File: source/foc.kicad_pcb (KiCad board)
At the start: 2 copper layers, 68.4 x 79 mm, 208 parts, among them J1 Conn_01x04_Male, J2 TYPE-C-31-M-12, P1 SWD, Q1 NCEP60T20, Q10 CSD19536KCS, Q11 CSD19536KCS, Q12 CSD19536KCS, Q2 CSD19536KCS, Q3 CSD19536KCS, Q4 CSD19536KCS, Q5 CSD19536KCS, Q6 CSD19536KCS, Q7 CSD19536KCS, Q8 CSD19536KCS, Q9 CSD19536KCS, U1 BMI160, U10 HT7550, U11 STM32F405RGT6, U12 AMS1117-3.3, U2 IRS21867S, U3 IRS21867S, U4 IRS21867S, U5 TX4130L/PW2902, U6 MS8311, U7 MS8311, U8 MS8311, U9 TJA1050T/CM,118, Y1 8MHz Crystal Resonator, X5032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

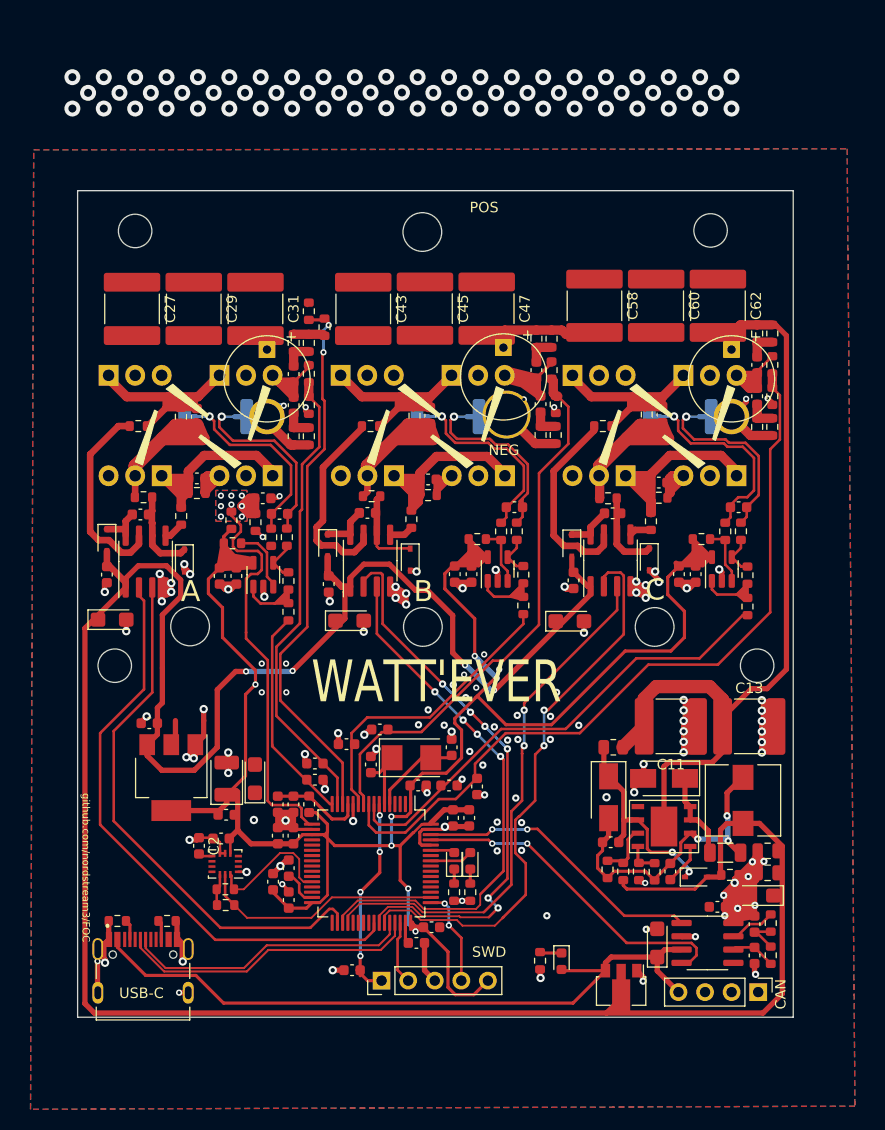
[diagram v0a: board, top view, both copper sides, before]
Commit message: Add files via upload
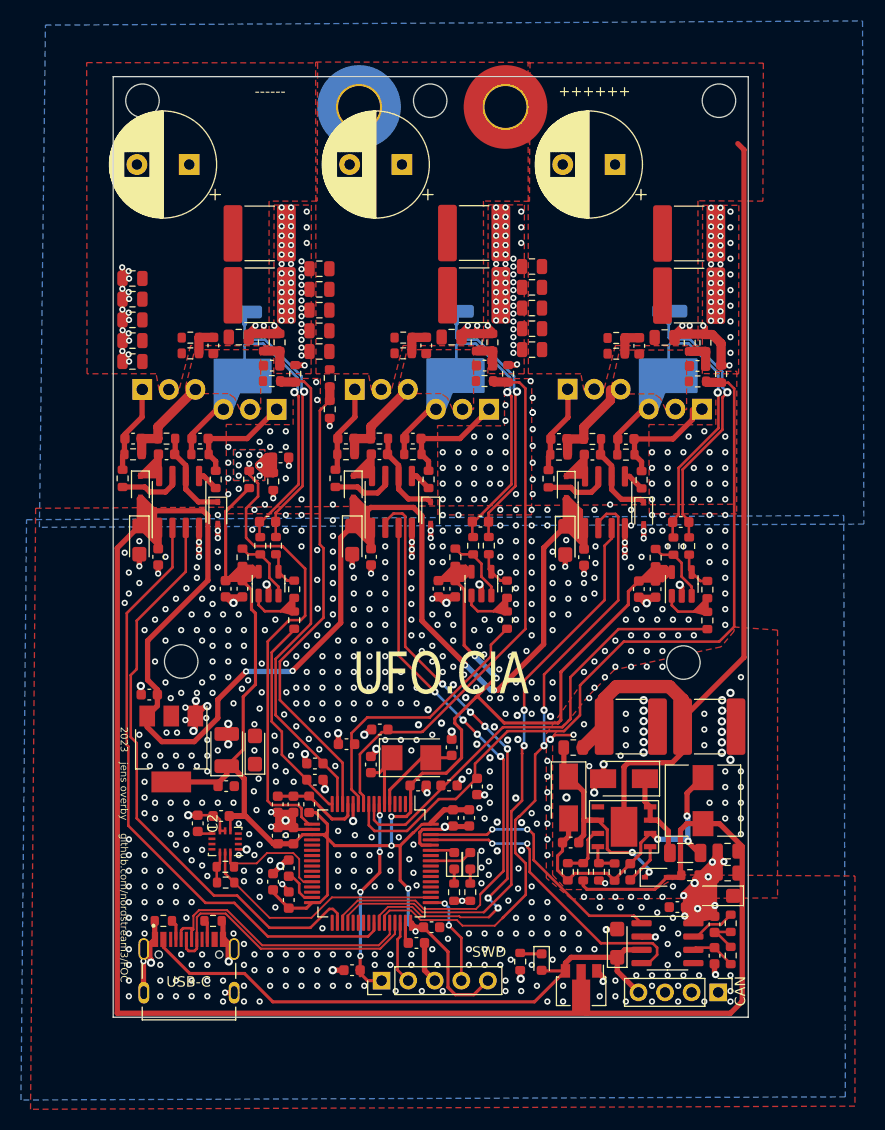
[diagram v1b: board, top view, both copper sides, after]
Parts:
- removed the C21 at (73.7, 108.8)
- removed the C22 at (75.3, 108.8)
- removed the C26 at (79.4, 102.9)
- removed the C31 at (77.1, 83.3)
- removed the C33 at (78.2, 87.5)
- removed the C40 at (93.8, 93.5)
- removed the C41 at (93.6, 99.6)
- removed the C58 at (109.5, 83.0)
- removed the H2 at (115.2, 113.7)
- removed the H4 at (70.8, 113.7)
- removed H8: MountingHole, MountingHole:MountingHole_3.7mm
- removed Q10, Q11, Q12, Q7, Q8, Q9: CSD19536KCS, Package_TO_SOT_THT:TO-220-3_Vertical
- removed the R21 at (80.2, 112.2)
- removed the R24 at (80.2, 109.3)
- removed the R25 at (74.9, 105.7)
- removed the R28 at (78.6, 105.1)
- removed the R29 at (80.1, 105.1)
- removed the U6 at (77.8, 108.7)
- added C27: 100n 100V, Capacitor_SMD:C_0805_2012Metric, F.Cu at (75.5, 86.0)
- added C28: 100n 100V, Capacitor_SMD:C_0805_2012Metric, F.Cu at (65.3, 88.3)
- added C29: 100n 100V, Capacitor_SMD:C_0805_2012Metric, F.Cu at (65.3, 86.3)
- added C30: 100n 100V, Capacitor_SMD:C_0805_2012Metric, F.Cu at (65.3, 80.4)
- added C32: 100n 100V, Capacitor_SMD:C_0805_2012Metric, F.Cu at (65.3, 82.4)
- added C34: 100n 100V, Capacitor_SMD:C_0805_2012Metric, F.Cu at (65.3, 84.3)
- added C35: 470u 80V, Capacitor_THT:CP_Radial_D10.0mm_P5.00mm, F.Cu at (70.8, 69.5)
- added C38: 2.2u, Capacitor_SMD:C_0603_1608Metric, F.Cu at (94.6, 110.0)
- added C39: 100n, Capacitor_SMD:C_0603_1608Metric, F.Cu at (96.2, 110.0)
- added C42: 2.2nF, Capacitor_SMD:C_0603_1608Metric, F.Cu at (85.7, 95.7)
- added C44: 100p, Capacitor_SMD:C_0603_1608Metric, F.Cu at (98.6, 103.6)
- added C46: 100n 100V, Capacitor_SMD:C_0805_2012Metric, F.Cu at (83.2, 87.4)
- added C48: 100n 100V, Capacitor_SMD:C_0805_2012Metric, F.Cu at (83.2, 79.5)
- added C54: 4.7n, Capacitor_SMD:C_0603_1608Metric, F.Cu at (93.4, 86.8)
- added C59: 2.2nF, Capacitor_SMD:C_0603_1608Metric, F.Cu at (106.1, 95.7)
- added C61: 100p, Capacitor_SMD:C_0603_1608Metric, F.Cu at (117.8, 103.7)
- added C63: 100n 100V, Capacitor_SMD:C_0805_2012Metric, F.Cu at (103.5, 85.2)
- added C67: 100n 100V, Capacitor_SMD:C_0805_2012Metric, F.Cu at (103.5, 81.2)
- added C68: 10u @ 100V, Capacitor_SMD:C_2220_5650Metric, F.Cu at (118.6, 76.1)
- added C69: 100n 100V, Capacitor_SMD:C_0805_2012Metric, F.Cu at (103.5, 83.2)
- added C70: 470u 80V, Capacitor_THT:CP_Radial_D10.0mm_P5.00mm, F.Cu at (111.5, 69.5)
- added C71: 4.7n, Capacitor_SMD:C_0603_1608Metric, F.Cu at (113.8, 86.8)
- added C72: 4.7n, Capacitor_SMD:C_0603_1608Metric, F.Cu at (119.4, 88.8)
- added H3: MountingHole, MountingHole:MountingHole_3.2mm_M3, F.Cu at (93.8, 63.4)
- added H7: MountingHole_Pad, MountingHole:MountingHole_4mm_Pad_TopOnly, F.Cu at (87.0, 64.0)
- added R35: 30k, Resistor_SMD:R_0603_1608Metric, F.Cu at (101.1, 113.0)
- added R39: 30k, Resistor_SMD:R_0603_1608Metric, F.Cu at (101.1, 110.1)
- added R41: 62k, Resistor_SMD:R_0603_1608Metric, F.Cu at (96.2, 107.0)
- added R44: 1k, Resistor_SMD:R_0603_1608Metric, F.Cu at (97.9, 105.9)
- added R45: 1k, Resistor_SMD:R_0603_1608Metric, F.Cu at (99.4, 105.9)
- added U7: MS8311, Package_TO_SOT_SMD:TSOT-23-5, F.Cu at (98.7, 109.6)
- C43, C60: value 10u @ 100V -> 2.2nF; footprint Capacitor_SMD:C_2220_5650Metric -> Capacitor_SMD:C_0603_1608Metric
- C45, C47, C62: value 10u @ 100V -> 100n 100V; footprint Capacitor_SMD:C_2220_5650Metric -> Capacitor_SMD:C_0805_2012Metric
- C49: value 470u 80V -> 10u @ 100V; footprint Custom:CP_Radial_D8.0mm_P5.00mm -> Capacitor_SMD:C_2220_5650Metric
- C50, C65: value 4.7n -> 100n 100V; footprint Capacitor_SMD:C_0603_1608Metric -> Capacitor_SMD:C_0805_2012Metric
- C51, C66: value 4.7n -> 10u @ 100V; footprint Capacitor_SMD:C_0603_1608Metric -> Capacitor_SMD:C_2220_5650Metric
- C52: value 2.2u -> 100n 100V; footprint Capacitor_SMD:C_0603_1608Metric -> Capacitor_SMD:C_0805_2012Metric
- C53: value 100n -> 470u 80V; footprint Capacitor_SMD:C_0603_1608Metric -> Capacitor_THT:CP_Radial_D10.0mm_P5.00mm
- C55: value 2.2nF -> 4.7n
- C56: value 2.2nF -> 2.2u
- C57: value 100p -> 100n
- C64: value 470u 80V -> 100n 100V; footprint Custom:CP_Radial_D8.0mm_P5.00mm -> Capacitor_SMD:C_0805_2012Metric
- H6: value MountingHole -> MountingHole_Pad; footprint MountingHole:MountingHole_3.7mm -> MountingHole:MountingHole_4mm_Pad_TopOnly
- moved H6 50.3 mm to (101.0, 64.0)
- moved C53 48.2 mm to (91.1, 69.5), turned to 180 degrees
- moved C52 42.6 mm to (83.2, 83.4), turned to 180 degrees
- moved Q4 31.9 mm to (99.4, 92.9)
- moved Q6 30.1 mm to (119.8, 92.9)
- moved C26 23.6 mm to (78.3, 103.6)
- moved Q3 23.6 mm to (86.6, 91.0)
- moved C65 23.5 mm to (103.5, 79.2), turned to 180 degrees
- moved R28 23.1 mm to (77.6, 105.9)
- moved R29 23.1 mm to (79.1, 105.9)
- moved R25 22.5 mm to (75.9, 107.0), turned to -90 degrees
- moved C50 22.1 mm to (83.2, 81.4), turned to 180 degrees
- moved C21 21.9 mm to (74.2, 110.1)
- moved C22 21.9 mm to (75.8, 110.1)
- moved R21 21.9 mm to (80.8, 113.0)
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- renumbered C36 to C21, C37 to C22, C42 to C26, C27 to C31, C29 to C33, C34 to C36, C35 to C37, C38 to C40, C39 to C41, C54 to C58, C67 to C73, C68 to C74, C69 to C75, C70 to C76, C71 to C77, C72 to C78, C73 to C79, C74 to C80, C75 to C81, C76 to C82, C77 to C83, C78 to C84, C79 to C85, C80 to C86, C81 to C87, C82 to C88, C83 to C89, C84 to C90, C85 to C91, C86 to C92, C87 to C93, C88 to C94, C89 to C95, C90 to C96, H3 to H2, H7 to H4, R35 to R21, R39 to R24, R41 to R25, R44 to R28, R45 to R29, U7 to U6
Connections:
- C26 pad 1: Net-(C42-Pad1) -> Net-(C26-Pad1)
- C26 pad 2: Net-(C42-Pad2) -> Net-(C26-Pad2)
- C43 pad 1: GND -> Net-(C43-Pad1)
- C43 pad 2: V_IN -> Net-(C43-Pad2)
- C45 pad 1: GND -> V_IN
- C45 pad 2: V_IN -> GND
- C47 pad 1: GND -> V_IN
- C47 pad 2: V_IN -> GND
- C49 pad 1: V_IN -> GND
- C49 pad 2: GND -> V_IN
- C50 pad 1: /driver/HS2 -> V_IN
- C50 pad 2: Net-(C50-Pad2) -> GND
- C51 pad 1: /driver/HS2 -> GND
- C51 pad 2: Net-(C51-Pad2) -> V_IN
- C52 pad 1: VCC -> V_IN
- C53 pad 1: VCC -> V_IN
- C55 pad 1: Net-(C55-Pad1) -> /driver/HS2
- C55 pad 2: /driver/HS3 -> Net-(C55-Pad2)
- C56 pad 1: Net-(C56-Pad1) -> VCC
- C56 pad 2: Net-(C56-Pad2) -> GND
- C57 pad 1: Net-(C57-Pad1) -> VCC
- C57 pad 2: Net-(C57-Pad2) -> GND
- C60 pad 1: GND -> Net-(C60-Pad1)
- C60 pad 2: V_IN -> Net-(C60-Pad2)
- C62 pad 1: GND -> V_IN
- C62 pad 2: V_IN -> GND
- C65 pad 1: /driver/HS3 -> V_IN
- C65 pad 2: Net-(C65-Pad2) -> GND
- C66 pad 1: /driver/HS3 -> GND
- C66 pad 2: Net-(C66-Pad2) -> V_IN
- NT3 pad 1: Net-(C42-Pad2) -> Net-(C44-Pad2)
- NT3 pad 2: Net-(C41-Pad2) -> Net-(C43-Pad2)
- NT4 pad 1: Net-(C42-Pad1) -> Net-(C44-Pad1)
- NT5 pad 1: Net-(C57-Pad2) -> Net-(C61-Pad2)
- NT5 pad 2: Net-(C56-Pad2) -> Net-(C60-Pad2)
- NT6 pad 1: Net-(C57-Pad1) -> Net-(C61-Pad1)
- Q3 pad 1: Net-(C24-Pad1) -> Net-(C42-Pad1)
- Q3 pad 3: /driver/HS1 -> /driver/HS2
- Q4 pad 1: Net-(C25-Pad1) -> Net-(C43-Pad1)
- Q4 pad 2: /driver/HS1 -> /driver/HS2
- Q4 pad 3: Net-(C25-Pad2) -> Net-(C43-Pad2)
- Q5 pad 1: Net-(C40-Pad1) -> Net-(C59-Pad1)
- Q5 pad 3: /driver/HS2 -> /driver/HS3
- Q6 pad 1: Net-(C41-Pad1) -> Net-(C60-Pad1)
- Q6 pad 2: /driver/HS2 -> /driver/HS3
- Q6 pad 3: Net-(C41-Pad2) -> Net-(C60-Pad2)
- R21 pad 2: /mcu/CURRENT_2 -> /mcu/CURRENT_1
- R28 pad 1: Net-(C42-Pad2) -> Net-(C26-Pad2)
- R29 pad 1: Net-(C42-Pad1) -> Net-(C26-Pad1)
- R37 pad 2: Net-(C40-Pad1) -> Net-(C42-Pad1)
- R38 pad 2: Net-(C41-Pad1) -> Net-(C43-Pad1)
- R42 pad 2: Net-(C40-Pad1) -> Net-(C42-Pad1)
- R43 pad 1: Net-(C41-Pad2) -> Net-(C43-Pad2)
- R43 pad 2: Net-(C41-Pad1) -> Net-(C43-Pad1)
- R46 pad 1: Net-(C41-Pad2) -> Net-(C43-Pad2)
- R47 pad 1: Net-(C50-Pad2) -> Net-(C54-Pad2)
- R48 pad 1: Net-(C51-Pad2) -> Net-(C55-Pad2)
- R49 pad 1: Net-(C50-Pad2) -> Net-(C54-Pad2)
- R50 pad 1: Net-(C51-Pad2) -> Net-(C55-Pad2)
- R52 pad 2: Net-(C55-Pad1) -> Net-(C59-Pad1)
- R53 pad 2: Net-(C56-Pad1) -> Net-(C60-Pad1)
- R56 pad 2: Net-(C55-Pad1) -> Net-(C59-Pad1)
- R57 pad 1: Net-(C56-Pad2) -> Net-(C60-Pad2)
- R57 pad 2: Net-(C56-Pad1) -> Net-(C60-Pad1)
- R58 pad 1: Net-(C57-Pad2) -> Net-(C61-Pad2)
- R59 pad 1: Net-(C57-Pad1) -> Net-(C61-Pad1)
- R60 pad 1: Net-(C56-Pad2) -> Net-(C60-Pad2)
- R61 pad 1: Net-(C65-Pad2) -> Net-(C71-Pad2)
- R62 pad 1: Net-(C66-Pad2) -> Net-(C72-Pad2)
- R63 pad 1: Net-(C65-Pad2) -> Net-(C71-Pad2)
- R64 pad 1: Net-(C66-Pad2) -> Net-(C72-Pad2)
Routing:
- net +12V: track 255.7 -> 295.1 mm, vias 8 -> 4
- net Net-(C41-Pad1): track 26.1 -> 0.00 mm
- net Net-(C61-Pad1): track 0.00 -> 25.9 mm, vias 0 -> 1
- net Net-(C61-Pad2): track 0.00 -> 25.6 mm
- net Net-(C44-Pad2): track 0.00 -> 25.4 mm, vias 0 -> 1
- net Net-(C44-Pad1): track 0.00 -> 25.0 mm, vias 0 -> 1
- net Net-(C40-Pad1): track 21.5 -> 0.00 mm
- net Net-(C55-Pad1): track 21.4 -> 0.00 mm
- net Net-(C56-Pad1): track 20.7 -> 0.00 mm
- net Net-(C57-Pad2): track 20.0 -> 0.00 mm, vias 1 -> 0
- net Net-(C42-Pad2): track 19.4 -> 0.00 mm, vias 1 -> 0
- net Net-(C57-Pad1): track 17.9 -> 0.00 mm, vias 1 -> 0
- net /driver/HS3: track 23.8 -> 9.21 mm
- net /driver/HS1: track 23.8 -> 9.78 mm
- net /driver/HO2: track 20.1 -> 6.19 mm
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- added copper zone on F.Cu, net /driver/HS1
- added copper zone on F.Cu, net /driver/HS2
- added copper zone on F.Cu, net /driver/HS3
- added copper zone on F.Cu, net V_IN
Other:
- board size 68.4 x 79 mm -> 60.7 x 89.9 mm
- board text added: "++++++"
- board text added: "------"
- board text added: "2023 jens overby github.com/nordstream3/FOC"
- board text added: "UFO.CIA"
- board text removed: "A"
- board text removed: "B"
- board text removed: "C"
- board text removed: "NEG"
- board text removed: "POS"
- board text removed: "WATT'EVER"
- board text removed: "github.com/nordstream3/FOC"
